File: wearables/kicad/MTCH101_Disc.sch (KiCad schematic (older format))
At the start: 15 parts, among them U1 MTCH101

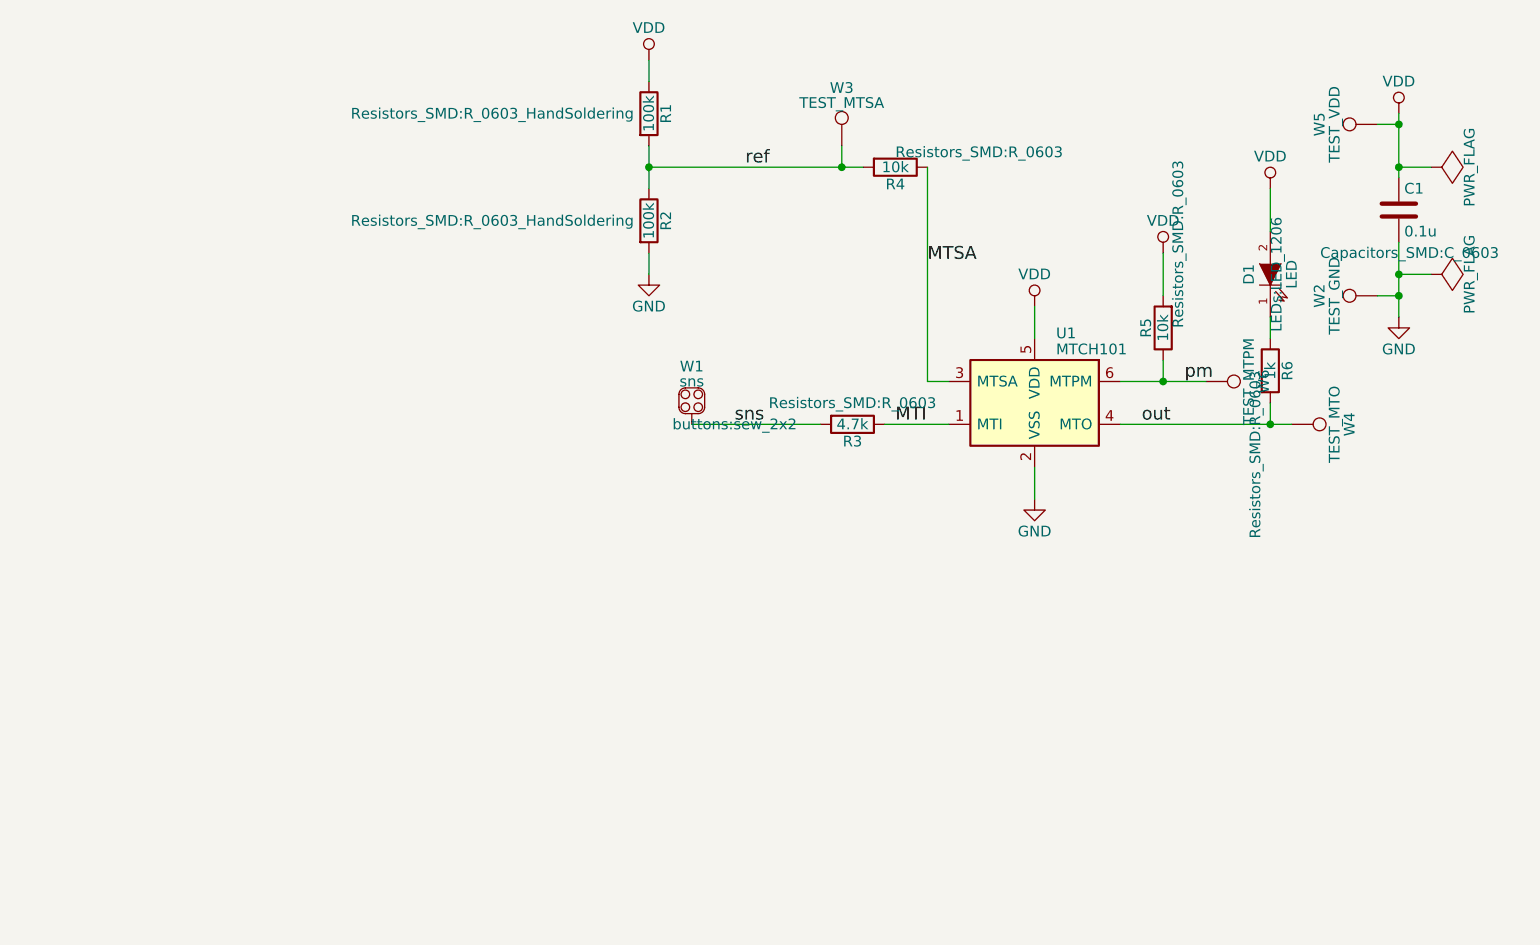
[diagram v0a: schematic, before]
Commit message: reworking.
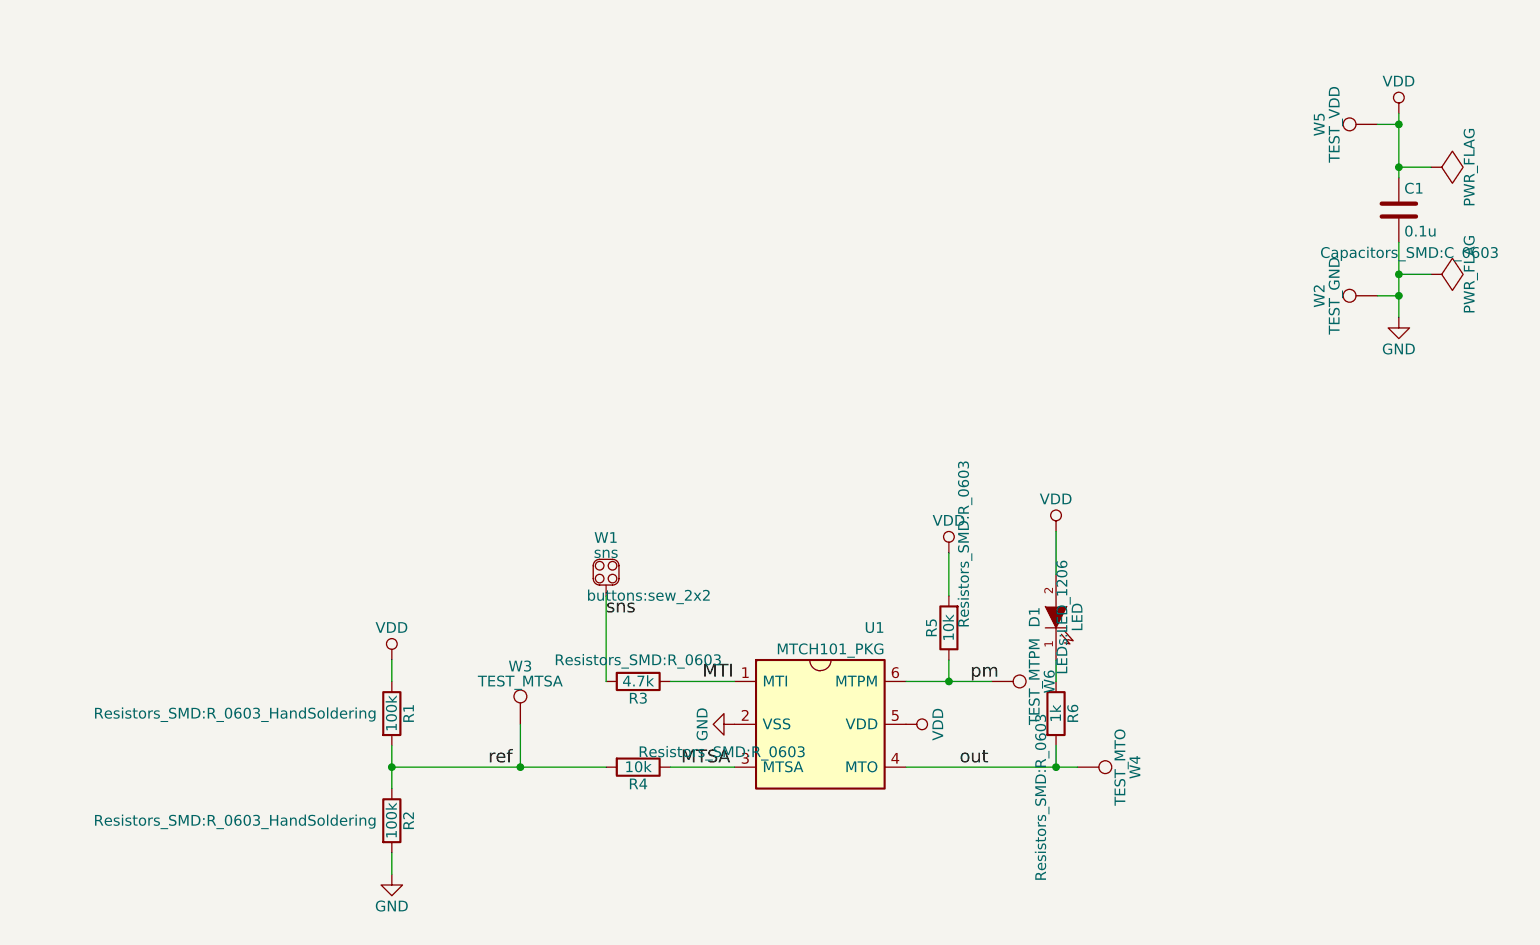
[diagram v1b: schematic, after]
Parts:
- removed U1: MTCH101, TO_SOT_Packages_SMD:SOT-23-6, symbol MTCH101
- added U1: MTCH101_PKG, TO_SOT_Packages_SMD:SOT-23-6, symbol MTCH101_PKG
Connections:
- net GND: now also U1.2 (VSS)
- net MTI: now also U1.1 (MTI)
- net MTSA: now also U1.3 (MTSA)
- net VDD: now also U1.5 (VDD)
- net out: now also U1.4 (MTO)
- net pm: now also U1.6 (MTPM)
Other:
- moved on the sheet: D1, R1, R2, R3, R4, R5, R6, W1, W3, W4, W6
